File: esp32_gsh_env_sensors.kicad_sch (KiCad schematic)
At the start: 45 parts, among them J1 USB_C_Receptacle_USB2.0, Q1 SS8050, Q2 SS8050, SW1 EN, SW2 BOOT, U1 MP2359, U2 CH340G, U3 ESP32-WROOM-32E, U4 MH-Z19B, U5 BME280, Y1 12MHz

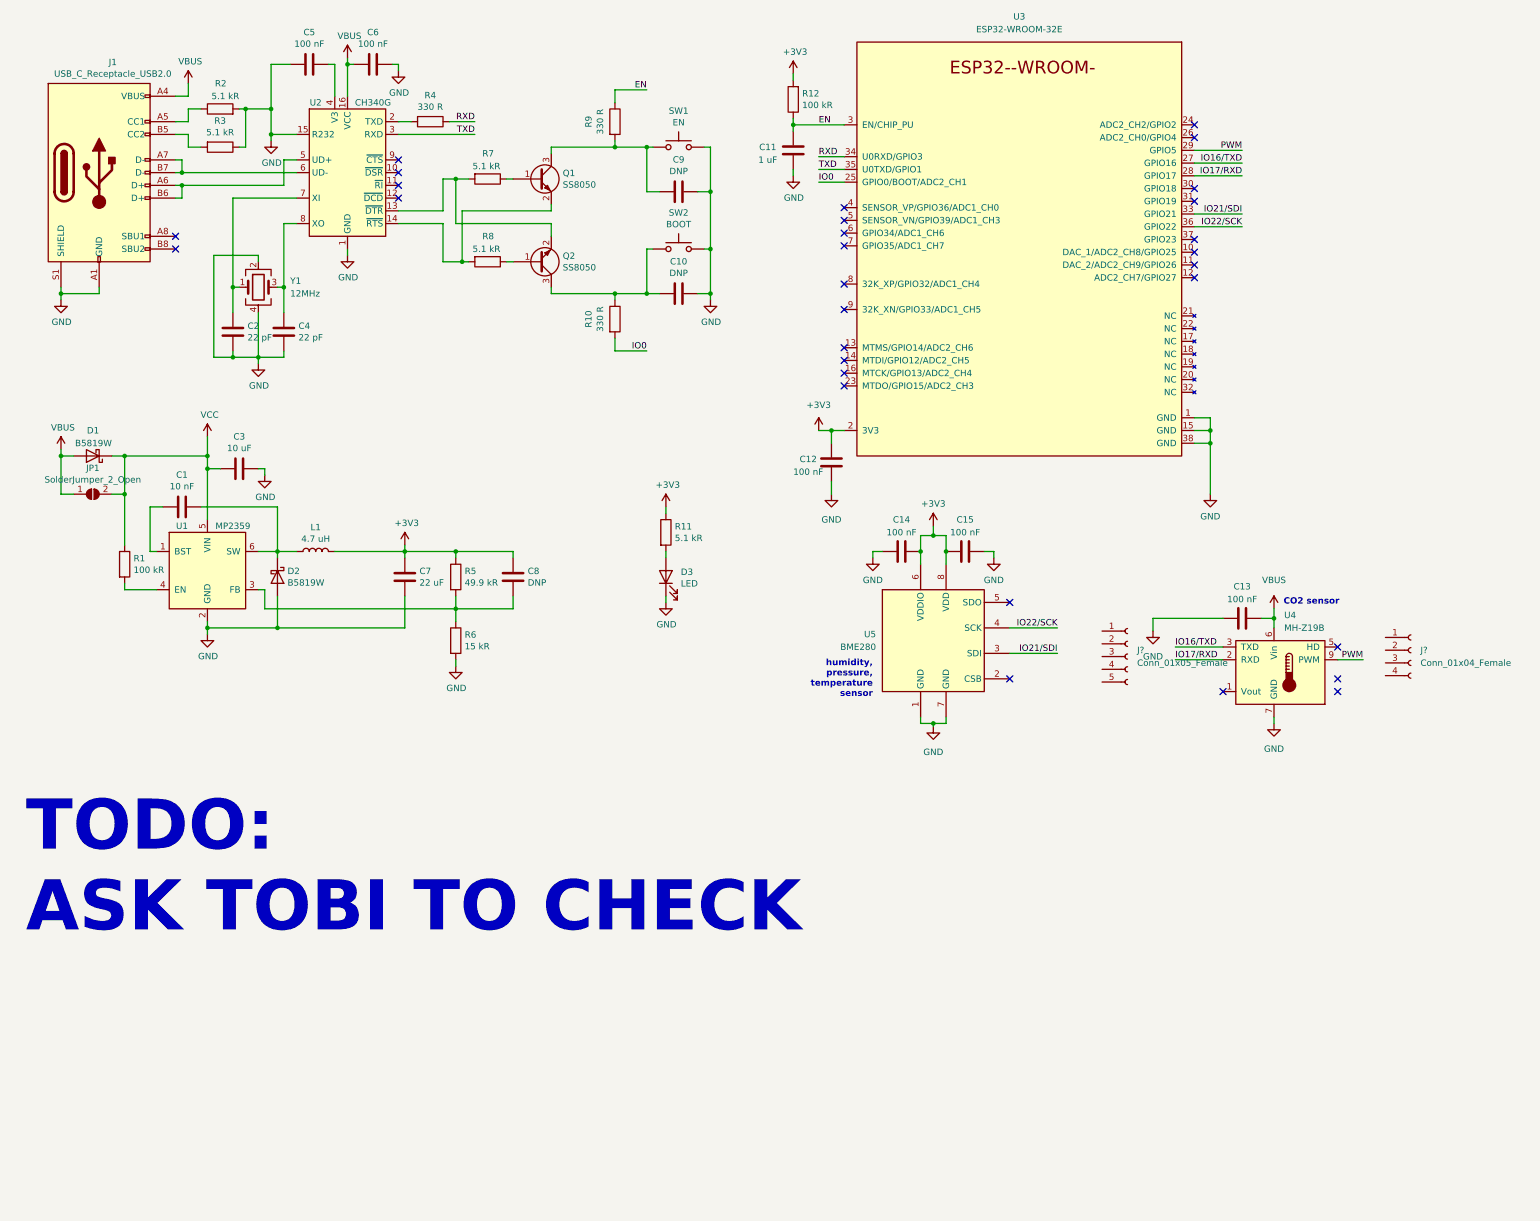
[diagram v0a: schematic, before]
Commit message: Update schematics
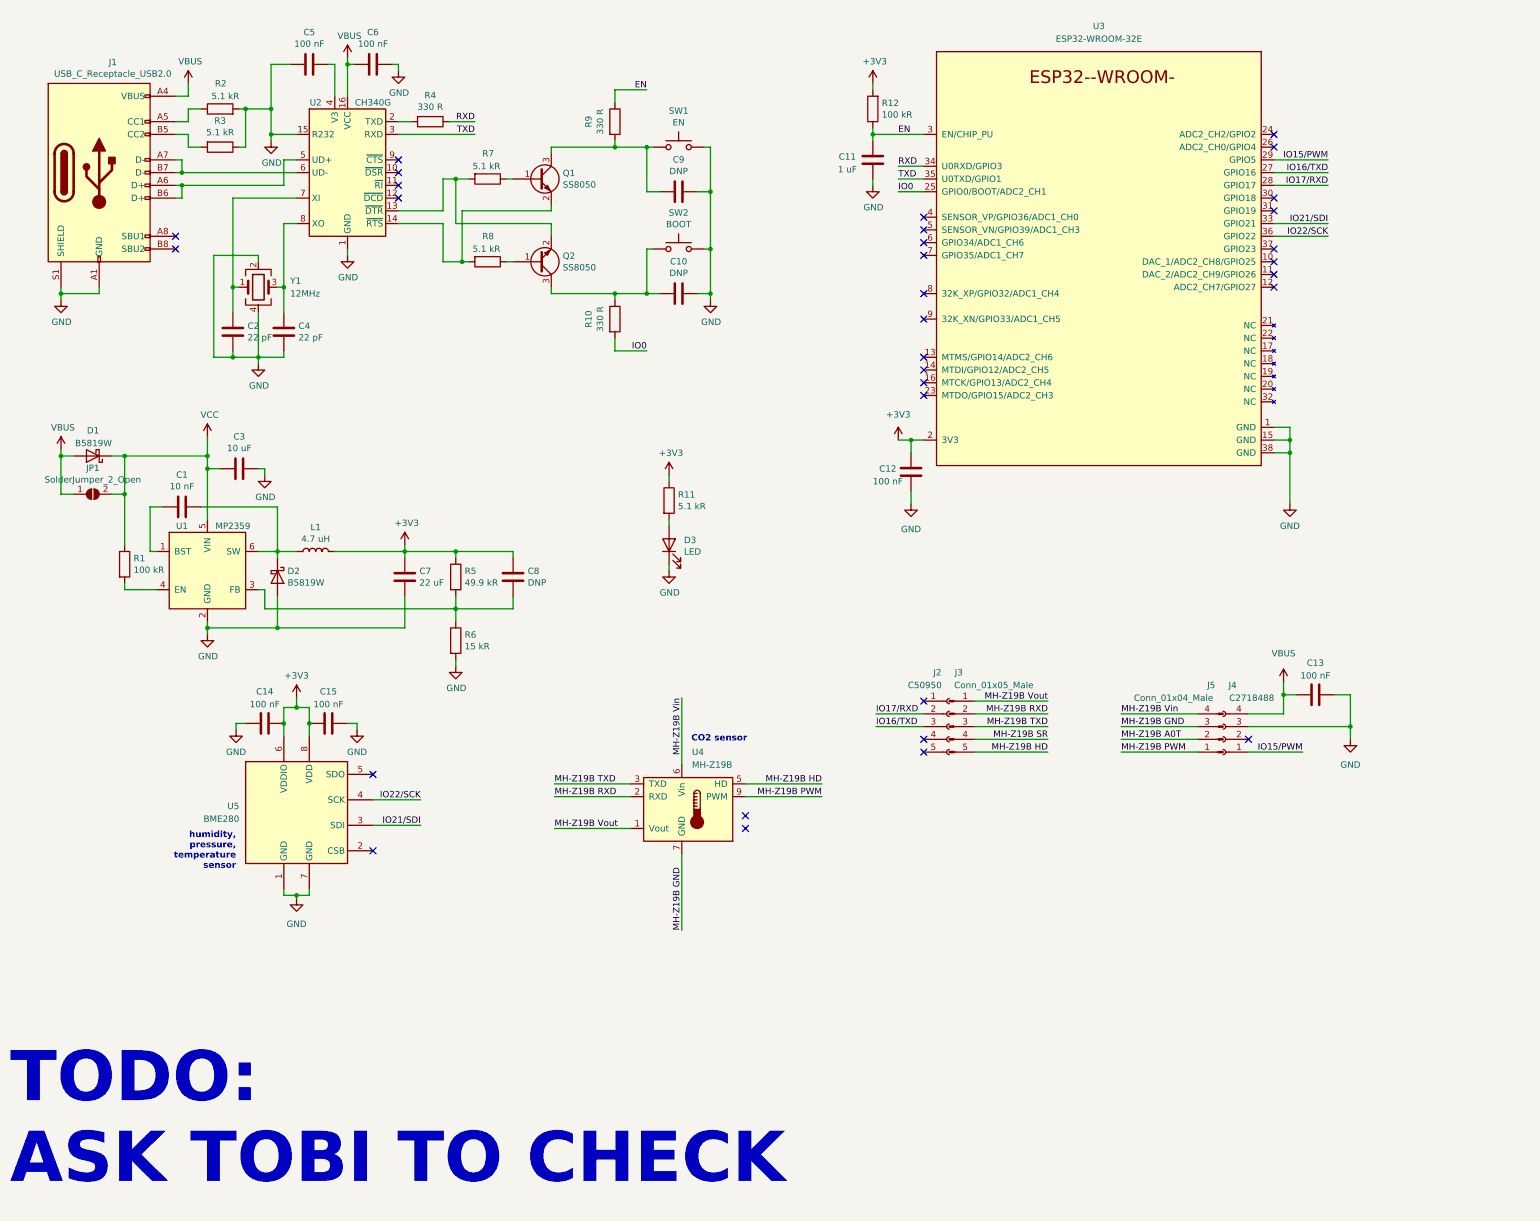
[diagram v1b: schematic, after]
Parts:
- added J3: Conn_01x05_Male, symbol Connector:Conn_01x05_Male
- added J5: Conn_01x04_Male, symbol Connector:Conn_01x04_Male
- J2: renamed from J?; value Conn_01x05_Female -> C50950
- J4: renamed from J?; value Conn_01x04_Female -> C2718488
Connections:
- net GND: now also C13.2, J4.3 (Pin_3); no longer C13.1, U4.7 (GND)
- net IO16/TXD: now also J2.3 (Pin_3); no longer U4.3 (TXD)
- net IO17/RXD: now also J2.2 (Pin_2); no longer U4.2 (RXD)
- net VBUS: now also C13.1, J4.4 (Pin_4); no longer C13.2, U4.6 (Vin)
- net MH-Z19B Vout: now reaches U4.1 (Vout)
- net MH-Z19B Vout: now also J3.1 (Pin_1)
- net MH-Z19B HD: now reaches U4.5 (HD)
- net MH-Z19B HD: now also J3.5 (Pin_5)
- net IO15/PWM: now reaches J4.1 (Pin_1)
- net IO15/PWM: now also U3.29 (GPIO5)
- net PWM renamed MH-Z19B PWM
- net MH-Z19B PWM: now also J5.1 (Pin_1); no longer U3.29 (GPIO5)
- new net MH-Z19B A0T: J5.2 (Pin_2)
- new net MH-Z19B GND: J5.3 (Pin_3), U4.7 (GND)
- new net MH-Z19B RXD: J3.2 (Pin_2), U4.2 (RXD)
- new net MH-Z19B SR: J3.4 (Pin_4)
- new net MH-Z19B TXD: J3.3 (Pin_3), U4.3 (TXD)
- new net MH-Z19B Vin: J5.4 (Pin_4), U4.6 (Vin)
- no-connect marks 30 -> 32
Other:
- moved on the sheet: C11, C12, C13, C14, C15, D3, J2, J4, R11, R12, U3, U4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
